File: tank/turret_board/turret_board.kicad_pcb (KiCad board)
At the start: 2 copper layers, 38 x 38.7 mm, 47 parts, among them J1 Conn_01x02_Male, J2 Conn_01x04_Male, J3 Conn_01x03_Male, J4 Conn_01x02_Male, J5 Conn_01x02_Male, Q1 2N3904, Q2 2N3904, U1 KA378R33, U2 pixart_ir, Y1 Crystal_4pin

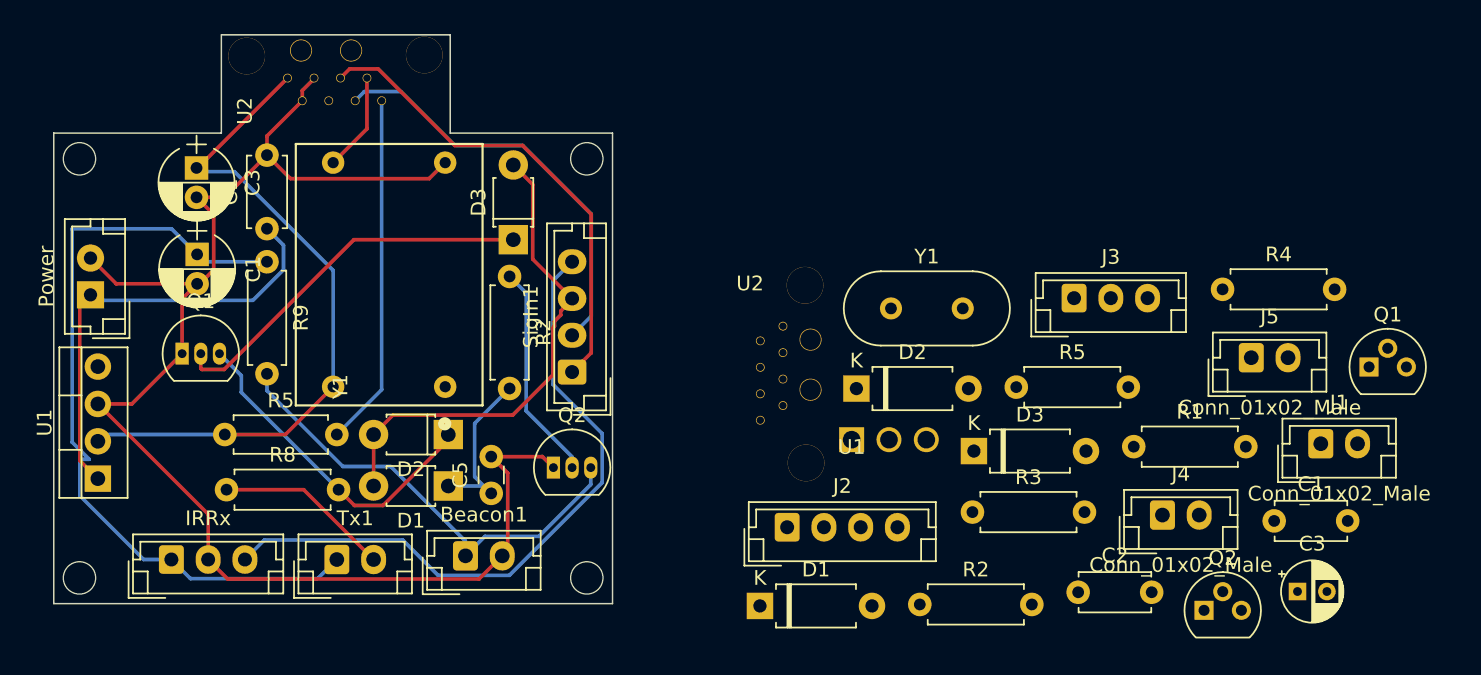
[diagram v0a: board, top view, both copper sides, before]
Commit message: revisions
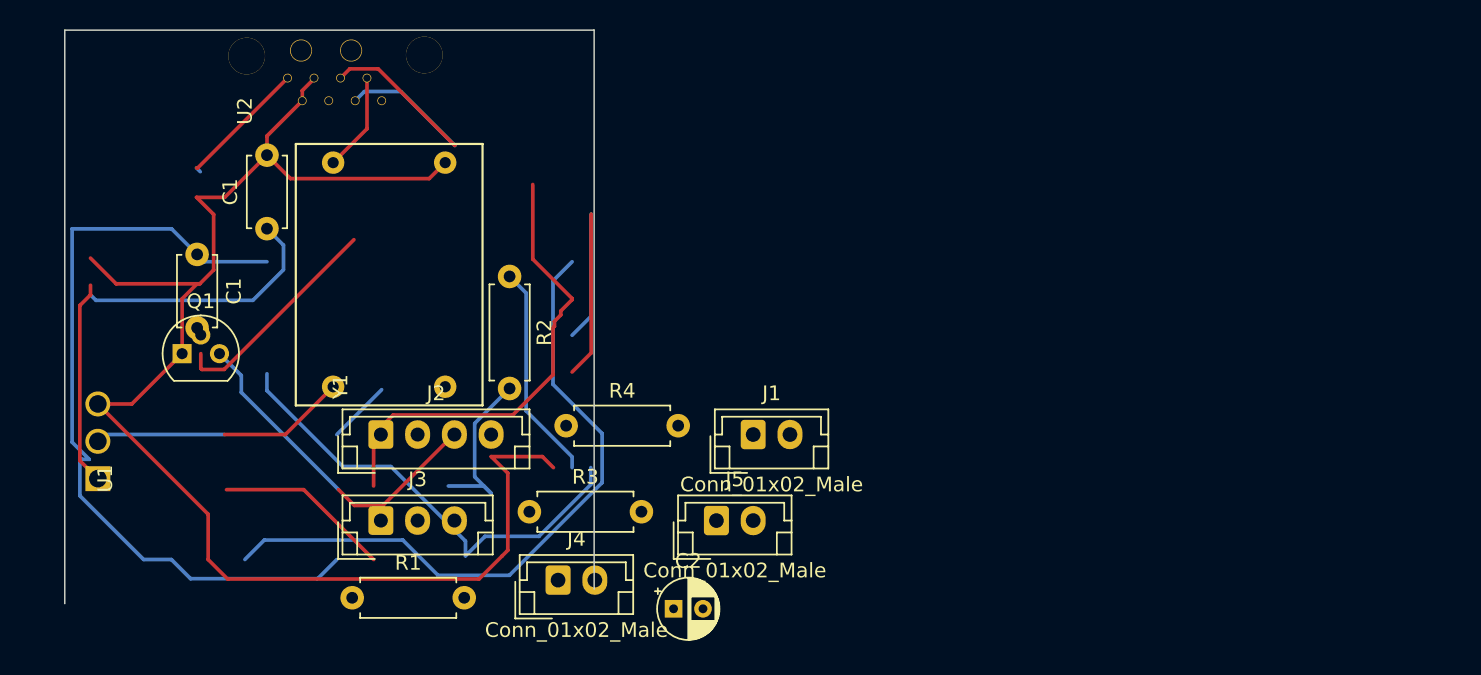
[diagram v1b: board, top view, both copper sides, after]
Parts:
- removed Beacon1: CONN_01X02, Connector_JST:JST_EH_B2B-EH-A_1x02_P2.50mm_Vertical
- removed the C1 at (265.7, 120.4)
- removed C3: CP, Capacitors_THT:CP_Radial_D5.0mm_P2.00mm
- removed C3: C, custom:CP_Radial_D4.0mm_P2.00mm
- removed C5: C, Capacitors_THT:C_Disc_D3.0mm_W1.6mm_P2.50mm
- removed D1, D2, D3: D, Diodes_THT:D_T-1_P5.08mm_Horizontal
- removed D1, D2, D3: D-Device, custom:D_A-405_P7.62mm_Horizontal
- removed G***: LOGO, modules:Tank
- removed IRRx: CONN_01X03, Connector_JST:JST_EH_B3B-EH-A_1x03_P2.50mm_Vertical
- removed Power: Conn_01x02_Male, JST:JST_EH_B02B-EH-A_02x2.50mm_Straight
- removed the Q1 at (272.2, 109.9)
- removed Q2: 2N3904, TO_SOT_Packages_THT:TO-92_Inline_Narrow_Oval
- removed Q2: 2N3904, custom:TO-92
- removed the R2 at (241.6, 126.1)
- removed R5, R9: R, Resistors_THT:R_Axial_DIN0207_L6.3mm_D2.5mm_P7.62mm_Horizontal
- removed R5: R, custom:R_Axial_DIN0207_L6.3mm_D2.5mm_P7.62mm_Horizontal
- removed R8: R, Resistor_THT:R_Axial_DIN0207_L6.3mm_D2.5mm_P7.62mm_Horizontal
- removed REF** (x4): MountingHole_2.2mm_M2, Mounting_Holes:MountingHole_2.2mm_M2
- removed SigIn1: CONN_01X04, Connector_JST:JST_EH_B4B-EH-A_1x04_P2.50mm_Vertical
- removed Tx1: TX, Connector_JST:JST_EH_B2B-EH-A_1x02_P2.50mm_Vertical
- removed the U1 at (237.0, 114.8)
- removed the U2 at (230.1, 103.7)
- removed the Y1 at (239.7, 105.9)
- C1: value CP -> C_Small; footprint Capacitors_THT:CP_Radial_D5.0mm_P2.00mm -> custom:C_Disc_D4.7mm_W2.5mm_P5.00mm
- C1: footprint Capacitor_THT:C_Disc_D4.7mm_W2.5mm_P5.00mm -> custom:C_Disc_D4.7mm_W2.5mm_P5.00mm
- C2: value C_Small -> C; footprint custom:C_Disc_D4.7mm_W2.5mm_P5.00mm -> custom:CP_Radial_D4.0mm_P2.00mm
- Q1: footprint TO_SOT_Packages_THT:TO-92_Inline_Narrow_Oval -> custom:TO-92
- R2: footprint Resistors_THT:R_Axial_DIN0207_L6.3mm_D2.5mm_P7.62mm_Horizontal -> custom:R_Axial_DIN0207_L6.3mm_D2.5mm_P7.62mm_Horizontal
- U1: footprint TO_SOT_Packages_THT:TO-220-4_Vertical -> custom:LM317T
- U2: footprint modules:pixart_ir -> custom:pixart_ir
- Y1: footprint Tank:ECS-100AX -> custom:ECS-100AX
- moved R1 54.1 mm to (203.0, 125.6)
- moved J3 49.5 mm to (205.0, 120.3)
- moved R4 45.6 mm to (217.6, 113.9)
- moved J4 41.3 mm to (217.0, 124.4)
- moved J1 38.6 mm to (230.3, 114.5)
- moved J5 38.0 mm to (227.8, 120.3)
- moved R3 30.1 mm to (215.1, 119.8)
- moved J2 28.3 mm to (205.0, 114.5)
- moved C2 27.5 mm to (224.9, 126.3)
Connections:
- C1 pad 1: 5V -> Net-(C1-Pad1)
- C2 pad 1: Net-(C2-Pad1) -> 3.3V
- J5 pad 2: GND -> 5V
- Q1 pad 2: Net-(D3-Pad1) -> IRSig
- Q1 pad 3: Net-(D2-Pad1) -> Net-(Q1-Pad3)
- R1 pad 1: Net-(Q2-Pad2) -> IRTx
- R1 pad 2: Net-(C2-Pad1) -> Net-(Q1-Pad3)
- R2 pad 1: Net-(Q2-Pad2) -> IRTx
- R2 pad 2: Net-(C5-Pad1) -> Net-(Q1-Pad3)
- R3 pad 1: IRTx -> 5V
- R3 pad 2: Net-(D1-Pad2) -> Beacon
- R4 pad 1: 5V -> 3.3V
- R4 pad 2: Beacon -> RESET
- U2 pad 4: Net-(U2-Pad4) -> unconnected-(U2-Pad4)
- Y1 pad 1: Net-(Y1-Pad1) -> unconnected-(Y1-Pad1)
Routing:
- net Net-(C1-Pad1): track 31.4 -> 85.1 mm
- net 5V: track 53.7 -> 0.00 mm
- net IRSig: track 33.8 -> 0.00 mm
- net IRRx: track 45.4 -> 77.4 mm
- net Net-(Q1-Pad3): track 0.00 -> 24.3 mm
- net 3.3V: track 46.3 -> 26.6 mm
- net RESET: track 24.0 -> 4.31 mm
- net IRTx: track 12.0 -> 26.7 mm
- net Net-(Q2-Pad2): track 14.8 -> 0.00 mm
- net Net-(D2-Pad1): track 22.7 -> 10.1 mm
- net Net-(C5-Pad1): track 11.7 -> 0.00 mm
- net SDA: track 28.5 -> 17.3 mm
- net SLC: track 32.7 -> 21.5 mm
- net Net-(D3-Pad1): track 25.9 -> 15.1 mm
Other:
- board size 38 x 38.7 mm -> 36 x 39 mm
- net class Default removed
